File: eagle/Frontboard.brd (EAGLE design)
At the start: 69.8 x 69.8 mm, 26 parts, among them IC1 LM35DM_NOPB

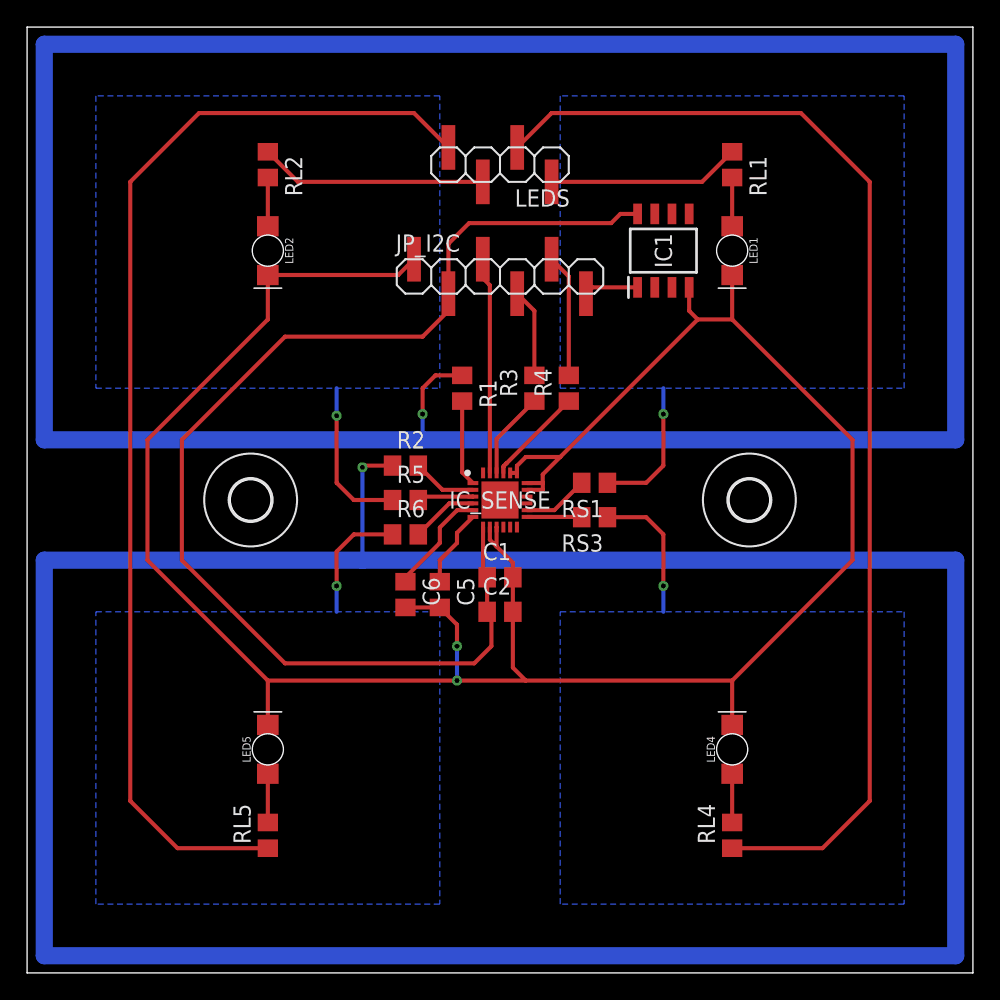
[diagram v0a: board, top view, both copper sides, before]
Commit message: updates
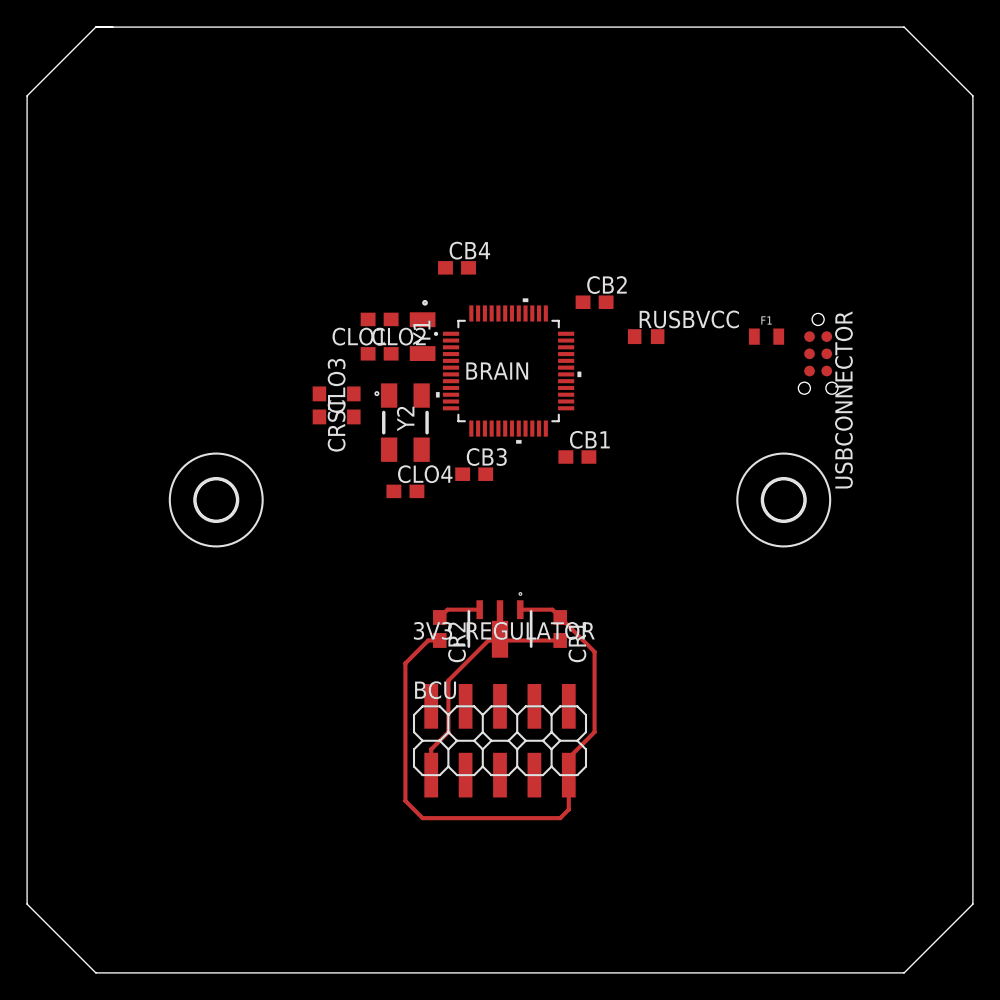
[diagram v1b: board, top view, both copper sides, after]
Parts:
- removed C1, C5: 0.1uf, rcl:C0805
- removed C2: 1uf, rcl:C0805
- removed C6: 2.2nf, rcl:C0805
- removed IC1: LM35DM_NOPB, LM35DM_NOPB:SOIC127P600X175-8N
- removed IC_SENSE: CY8CMBR3116-LQXIT, CY8CMBR3116-LQXIT:QFN50P400X400X60-25N
- removed JP_I2C: I2C, pinhead:1X06SMD
- removed LED1, LED2, LED4, LED5: WHITE, SparkFun-LED:LED-1206-BOTTOM
- removed LEDS: LEDS, pinhead:1X04SMD
- removed R1, R2, R5, R6, RS1, RS3: 560E, resistor:R0805
- removed R3, R4, RL1, RL2, RL4, RL5: 330E, resistor:R0805
- added 3V3_REGULATOR: MCP1703T-3302E_MB, MCP1703T-3302E_MB:SOT-89(MB)
- added BCU: BCU, pinhead:2X05SMD
- added BRAIN: STM32L072CBT, STM32L072CBT:LQFP48-7X7MM
- added CB1, CB2, CB3, CB4: 100nf, rcl:C0603
- added CLO1: 7pF, rcl:C0603
- added CLO2: 7pf, rcl:C0603
- added CLO3, CLO4: 18pf, rcl:C0603
- added CR1, CR2: 1uF, rcl:C0603
- added CRST: 0.1uF, rcl:C0603
- added F1: PPTC_6V500MA, SparkFun-Fuses:0805
- added RUSBVCC: 220, resistor:R0603
- added USBCONNECTOR: (no value), tag-connect:TC2030-MCP-NL
- added Y1: ABS07-32.768KHZ-7-T, ABS07-32.768KHZ-7-T:ABS-07
- added Y2: ABM3B-8.000MHZ-B2-T, ABM3B-8.000MHZ-B2-T:ABM3B
- moved U$1 2.54 mm to (14.0, 34.9)
- moved U$2 2.54 mm to (55.9, 34.9)
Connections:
- removed net HOST_INT: IC_SENSE.23, JP_I2C.3
- removed net I2C_SCL: JP_I2C.4, R3.2
- removed net I2C_SDA: JP_I2C.5, R4.2
- removed net LED1: LEDS.1, RL1.1
- removed net LED2: LEDS.3, RL2.1
- removed net LED4: LEDS.2, RL4.1
- removed net LED5: LEDS.4, RL5.1
- removed net N$14: LED5.A, RL5.2
- removed net N$15: LED4.A, RL4.2
- removed net N$16: LED2.A, RL2.2
- removed net N$17: LED1.A, RL1.2
- removed net N$19: C5.1, IC_SENSE.6
- removed net N$20: C6.1, IC_SENSE.5
- removed net N$4: IC_SENSE.13, RS3.2
- removed net N$5: IC_SENSE.1, R1.2
- removed net N$6: IC_SENSE.2, R2.2
- removed net N$7: IC_SENSE.4, R6.2
- removed net N$8: IC_SENSE.3, R5.2
- removed net SENS_1: RS1.1
- removed net SENS_2: R5.1
- removed net SENS_3: RS3.1
- removed net SENS_4: R6.1
- removed net SENS_PROX_1: R1.1
- removed net SENS_PROX_2: R2.1
- removed net TEMP: IC1.1, JP_I2C.6
- removed net VCC: C1.1, C2.1, IC1.8, IC_SENSE.7, JP_I2C.2
- new net +3V3: 3V3_REGULATOR.3, BRAIN.1, BRAIN.24, BRAIN.48, BRAIN.9, CB1.1, CB2.1, CB3.1, CB4.1, CR2.1
- new net +5V: 3V3_REGULATOR.2, 3V3_REGULATOR.4, BCU.1, CR1.2
- new net OSC32_IN: BRAIN.3, CLO1.2, Y1.1
- new net OSC32_OUT: BRAIN.4, CLO2.2, Y1.2
- new net OSC_IN: BRAIN.5, CLO3.2, Y2.1
- new net OSC_OUT: BRAIN.6, CLO4.2, Y2.3
- new net PA10: BRAIN.31
- new net PB3: BRAIN.39
- new net PB4: BRAIN.40
- new net RXD: BCU.7
- new net TXD: BCU.3
- new net USB_DM: BRAIN.32, USBCONNECTOR.5
- new net USB_DP: BRAIN.33, USBCONNECTOR.4
- new net USB_VCC: BRAIN.36, RUSBVCC.1
- net GND: now also 3V3_REGULATOR.1, BCU.9, BRAIN.23, BRAIN.35, BRAIN.47, BRAIN.8, CB1.2, CB2.2, CB3.2, CB4.2, CLO1.1, CLO2.1, CLO3.1, CLO4.1, CR1.1, CR2.2, CRST.2, USBCONNECTOR.3, Y2.2, Y2.4; no longer C1.2, C2.2, C5.2, C6.2, IC1.4, IC_SENSE.17, IC_SENSE.18, IC_SENSE.19, IC_SENSE.20, IC_SENSE.8, IC_SENSE.9, JP_I2C.1, LED1.C, LED2.C, LED4.C, LED5.C
- net N$1: now also BRAIN.7, CRST.1; no longer IC_SENSE.22, R3.1
- net N$2: now also F1.2, USBCONNECTOR.2; no longer IC_SENSE.21, R4.1
- net N$3: now also F1.1, RUSBVCC.2; no longer IC_SENSE.14, RS1.2
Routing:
- net SENS_PROX_2: track 202.3 -> 0.00 mm, vias 1 -> 0
- net SENS_PROX_1: track 200.2 -> 0.00 mm, vias 1 -> 0
- net GND: track 178.5 -> 45.5 mm, vias 2 -> 0
- net VCC: track 88.9 -> 0.00 mm
- net LED4: track 86.5 -> 0.00 mm
- net LED5: track 84.0 -> 0.00 mm
- net +5V: track 0.00 -> 19.2 mm
- net LED2: track 16.8 -> 0.00 mm
- net HOST_INT: track 16.0 -> 0.00 mm
- net LED1: track 14.3 -> 0.00 mm
- net SENS_2: track 11.6 -> 0.00 mm, vias 1 -> 0
- net SENS_3: track 10.4 -> 0.00 mm, vias 1 -> 0
- net SENS_1: track 10.4 -> 0.00 mm, vias 1 -> 0
- net I2C_SDA: track 9.10 -> 0.00 mm
- net SENS_4: track 9.10 -> 0.00 mm, vias 1 -> 0
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- removed copper zone on layer 16, net SENS_1
- removed copper zone on layer 16, net SENS_2
- removed copper zone on layer 16, net SENS_3
- removed copper zone on layer 16, net SENS_4
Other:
- outline, holes or cut-outs redrawn

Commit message: updates
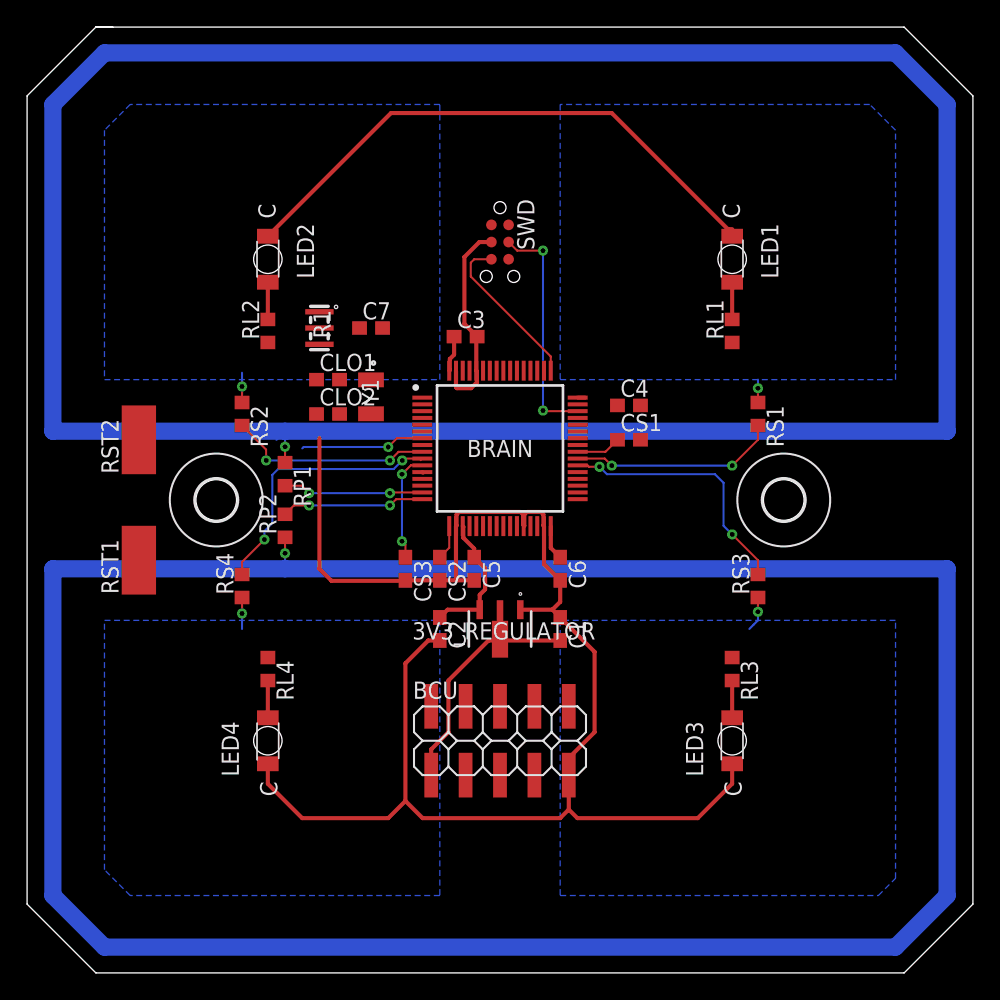
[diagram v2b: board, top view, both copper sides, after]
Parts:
- removed CB1, CB2, CB3, CB4: 100nf, rcl:C0603
- removed CLO3, CLO4: 18pf, rcl:C0603
- removed CRST: 0.1uF, rcl:C0603
- removed F1: PPTC_6V500MA, SparkFun-Fuses:0805
- removed RUSBVCC: 220, resistor:R0603
- removed USBCONNECTOR: (no value), tag-connect:TC2030-MCP-NL
- removed Y2: ABM3B-8.000MHZ-B2-T, ABM3B-8.000MHZ-B2-T:ABM3B
- added C3, C4, C5, C6: 100nf, rcl:C0603
- added C7: 0.1uF, rcl:C0603
- added CS1, CS2, CS3: 47nF, rcl:C0603
- added LED1, LED2, LED3, LED4: WL-SMRW156120BS75300-B_RVS-MOUNT, Wurth_Elektronik_Optoelectronics_rev15b (1):WL-SMRW-1206-CYLDR-REVERSE-MOUNT
- added R1: CSTCE8M00G55-R0, CSTCE8M00G55-R0:CSTCE12M0G55-R0
- added RL1, RL2, RL3, RL4, RP1, RP2, RS1, RS2, RS3, RS4: 330E, rcl:R0603
- added RST1, RST2: 0, wirepad:SMD2,54-5,08
- added SWD: SWD, tag-connect:TC2030-MCP-NL
- BRAIN: value STM32L072CBT -> STM32L152RET6; device STM32L072CBT:LQFP48-7X7MM -> STM32L152RET6:QFP50P1200X1200X160-64N
- moved Y1 5.85 mm to (25.4, 42.5)
- moved CLO1 5.85 mm to (22.2, 43.8), turned to 0 degrees
- moved CLO2 5.85 mm to (22.2, 41.3)
- moved BRAIN 5.75 mm to (34.9, 38.7)
- renumbered CR1 to C1, CR2 to C2
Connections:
- removed net PA10: BRAIN.31
- removed net PB3: BRAIN.39
- removed net PB4: BRAIN.40
- removed net USB_DM: BRAIN.32, USBCONNECTOR.5
- removed net USB_DP: BRAIN.33, USBCONNECTOR.4
- removed net USB_VCC: BRAIN.36, RUSBVCC.1
- new net G10_IO1: BRAIN.37
- new net G10_IO2: BRAIN.38, RS3.2
- new net G10_IO3: BRAIN.39, RS1.2
- new net G10_IO4: BRAIN.40, CS1.1
- new net G1_IO1: BRAIN.14
- new net G1_IO2: BRAIN.15, RP1.2
- new net G1_IO3: BRAIN.16, RP2.2
- new net G1_IO4: BRAIN.17, CS2.1
- new net G7_IO1: BRAIN.33
- new net G7_IO2: BRAIN.34
- new net G7_IO3: BRAIN.35
- new net G7_IO4: BRAIN.36
- new net G8_IO1: BRAIN.8
- new net G8_IO2: BRAIN.9, RS2.2
- new net G8_IO3: BRAIN.10, RS4.2
- new net G8_IO4: BRAIN.11, CS3.1
- new net I2C1_SCL: BRAIN.58
- new net I2C1_SDA: BRAIN.59
- new net LED1: RL1.1
- new net LED2: RL2.1
- new net LED4: RL3.1
- new net LED5: RL4.1
- new net N$10: BRAIN.45
- new net N$19: LED1.2, RL1.2
- new net N$20: LED2.2, RL2.2
- new net N$21: LED3.2, RL3.2
- new net N$22: LED4.2, RL4.2
- new net N$7: BRAIN.42
- new net N$8: BRAIN.43
- new net N$9: BRAIN.44
- new net NRST: BRAIN.7, C7.1, RST1.1, SWD.1
- new net SENS_1: RS1.1
- new net SENS_2: RS2.1
- new net SENS_3: RS3.1
- new net SENS_4: RS4.1
- new net SENS_PROX_1: RP1.1
- new net SENS_PROX_2: RP2.1
- new net SWCLK: BRAIN.49, SWD.5
- new net SWDIO: BRAIN.46, SWD.4
- new net VDD: SWD.2
- new net VLCD: BRAIN.1
- net +3V3: now also BRAIN.13, BRAIN.19, BRAIN.32, BRAIN.64, C3.1, C4.1, C5.1, C6.1; no longer BRAIN.1, BRAIN.24, BRAIN.9, CB1.1, CB2.1, CB3.1, CB4.1
- net GND: now also BRAIN.12, BRAIN.18, BRAIN.28, BRAIN.31, BRAIN.60, BRAIN.63, C3.2, C4.2, C5.2, C6.2, C7.2, CS1.2, CS2.2, CS3.2, LED1.1, LED2.1, LED3.1, LED4.1, R1.2, RST2.1, SWD.3; no longer BRAIN.23, BRAIN.35, BRAIN.8, CB1.2, CB2.2, CB3.2, CB4.2, CLO3.1, CLO4.1, CRST.2, USBCONNECTOR.3, Y2.2, Y2.4
- net N$1: now also BRAIN.55; no longer BRAIN.7, CRST.1
- net N$2: now also BRAIN.56; no longer F1.2, USBCONNECTOR.2
- net N$3: now also BRAIN.41; no longer F1.1, RUSBVCC.2
- net OSC_IN: now also R1.1; no longer CLO3.2, Y2.1
- net OSC_OUT: now also R1.3; no longer CLO4.2, Y2.3
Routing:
- net SENS_PROX_1: track 0.00 -> 186.7 mm, vias 0 -> 1
- net SENS_PROX_2: track 0.00 -> 185.8 mm, vias 0 -> 1
- net GND: track 45.5 -> 172.3 mm
- net G8_IO3: track 0.00 -> 20.0 mm, vias 0 -> 2
- net G10_IO2: track 0.00 -> 19.1 mm, vias 0 -> 2
- net SWDIO: track 0.00 -> 17.2 mm, vias 0 -> 2
- net G10_IO3: track 0.00 -> 15.4 mm, vias 0 -> 2
- net G8_IO2: track 0.00 -> 15.1 mm, vias 0 -> 2
- net +3V3: track 3.18 -> 16.0 mm
- net SWCLK: track 0.00 -> 12.1 mm
- net G1_IO3: track 0.00 -> 10.6 mm, vias 0 -> 2
- net G1_IO2: track 0.00 -> 10.4 mm, vias 0 -> 2
- net NRST: track 0.00 -> 9.19 mm, vias 0 -> 1
- net G8_IO4: track 0.00 -> 8.01 mm, vias 0 -> 2
- net G10_IO4: track 0.00 -> 3.30 mm
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- added copper zone on layer 16, net SENS_1
- added copper zone on layer 16, net SENS_2
- added copper zone on layer 16, net SENS_3
- added copper zone on layer 16, net SENS_4
